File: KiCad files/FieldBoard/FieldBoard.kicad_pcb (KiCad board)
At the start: 2 copper layers, 150 x 150 mm, 146 parts, among them U1 TTP223-BA6, U10 TTP223-BA6, U11 TTP223-BA6, U12 TTP223-BA6, U2 TTP223-BA6, U3 TTP223-BA6, U4 TTP223-BA6, U5 TTP223-BA6, U6 TTP223-BA6, U7 TTP223-BA6, U8 TTP223-BA6, U9 TTP223-BA6

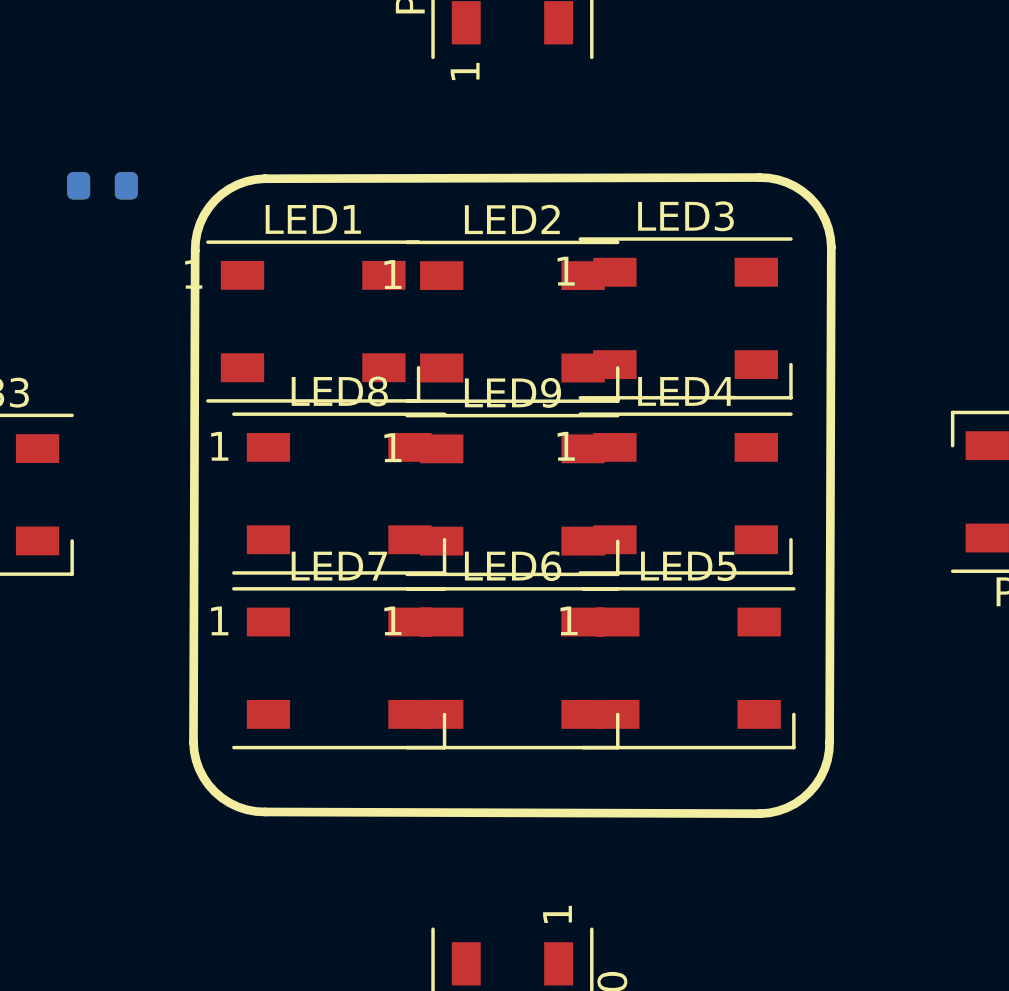
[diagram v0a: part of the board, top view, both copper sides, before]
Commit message: update
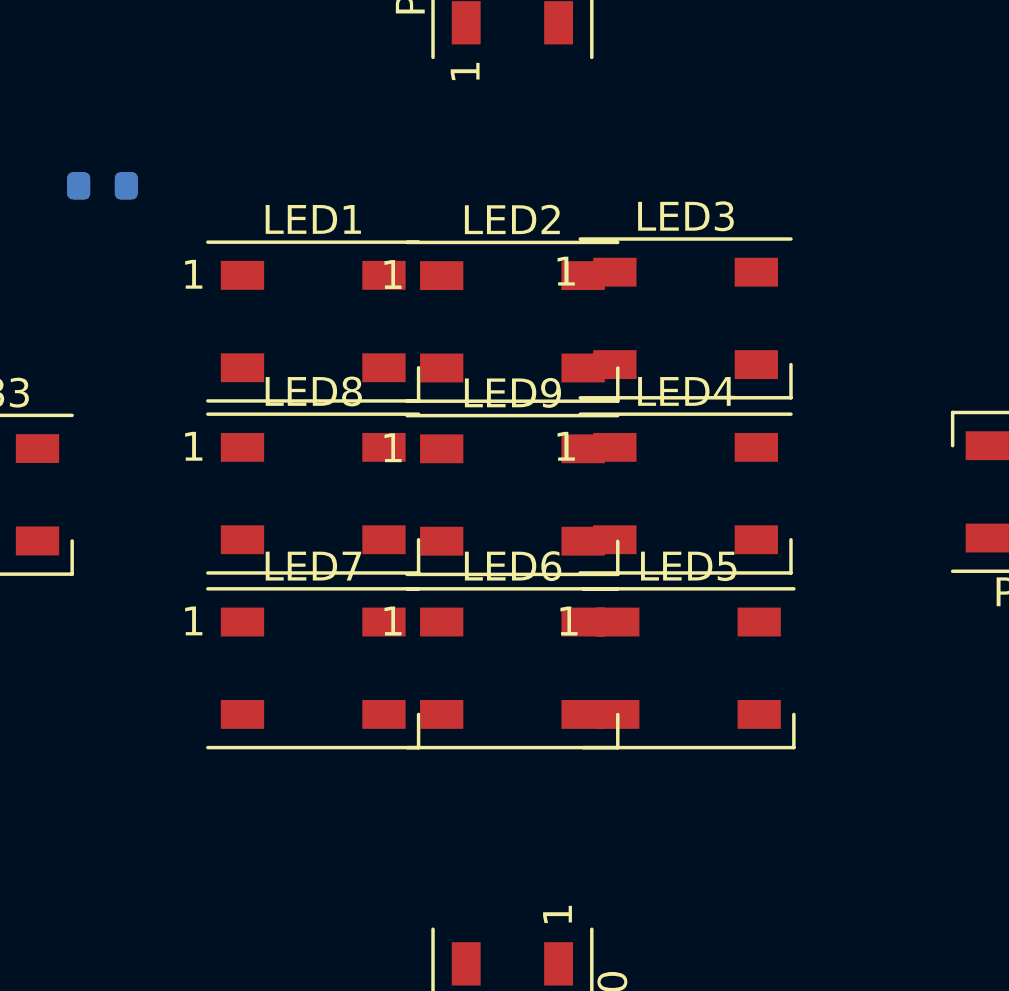
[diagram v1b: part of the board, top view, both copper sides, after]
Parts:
- moved LED7 0.90 mm to (136.9, 95.6)
- moved LED8 0.90 mm to (136.9, 89.6)
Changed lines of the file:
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@@
   )
   (footprint "LED_SMD:LED_WS2812B_PLCC4_5.0x5.0mm_P3.2mm" (layer "F.Cu")
-    (at 137.800004 95.608851)
+    (at 136.9 95.608851)
     (descr "https://cdn-shop.adafruit.com/datasheets/WS2812B.pdf")
     (tags "LED RGB NeoPixel")
@@
   )
   (footprint "LED_SMD:LED_WS2812B_PLCC4_5.0x5.0mm_P3.2mm" (layer "F.Cu")
-    (at 137.800004 89.558851)
+    (at 136.9 89.558851)
     (descr "https://cdn-shop.adafruit.com/datasheets/WS2812B.pdf")
     (tags "LED RGB NeoPixel")
@@
     )
   )
-  (gr_arc (start 154.788425 98.154422) (mid 154.1 99.9) (end 152.3789 100.647521) (layer "F.SilkS") (width 0.3))
   (gr_arc (start 78.9 66.5) (mid 82.435534 67.964466) (end 83.9 71.5) (layer "F.SilkS") (width 0.3))
-  (gr_line (start 154.847521 81.0211) (end 154.788425 98.154422) (layer "F.SilkS") (width 0.3))
-  (gr_arc (start 152.354422 78.611575) (mid 154.1 79.3) (end 154.847521 81.0211) (layer "F.SilkS") (width 0.3))
-  (gr_arc (start 135.245578 100.588425) (mid 133.5 99.9) (end 132.752479 98.1789) (layer "F.SilkS") (width 0.3))
   (gr_line (start 69.1 113.1) (end 78.9 113.064466) (layer "F.SilkS") (width 0.3))
-  (gr_line (start 135.2211 78.652479) (end 152.354422 78.611575) (layer "F.SilkS") (width 0.3))
   (gr_line (start 78.9 66.5) (end 69.1 66.5) (layer "F.SilkS") (width 0.3))
   (gr_arc (start 83.9 108.064466) (mid 82.435534 111.6) (end 78.9 113.064466) (layer "F.SilkS") (width 0.3))
-  (gr_arc (start 132.811575 81.145578) (mid 133.5 79.4) (end 135.2211 78.652479) (layer "F.SilkS") (width 0.3))
   (gr_line (start 83.9 108.064466) (end 83.9 71.5) (layer "F.SilkS") (width 0.3))
-  (gr_line (start 135.245578 100.588425) (end 152.3789 100.647521) (layer "F.SilkS") (width 0.3))
-  (gr_line (start 132.811575 81.145578) (end 132.752479 98.1789) (layer "F.SilkS") (width 0.3))
   (gr_arc (start 68.857864 34.657864) (mid 74.715728 20.515728) (end 88.857864 14.657864) (layer "Edge.Cuts") (width 0.1))
   (gr_arc (start 218.857864 144.657864) (mid 213 158.8) (end 198.857864 164.657864) (layer "Edge.Cuts") (width 0.1))
